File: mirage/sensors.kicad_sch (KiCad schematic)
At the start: 22 parts, among them U2 ADXL375BCCZ-RL7, U3 TMP275AIDGKR VSSOP8, U4 MS5607-02BA, U5 BMI088, U6 TMP275AIDGKR VSSOP8, U7 TMP275AIDGKR VSSOP8, U8 TMP275AIDGKR VSSOP8, U9 MMC5983MA

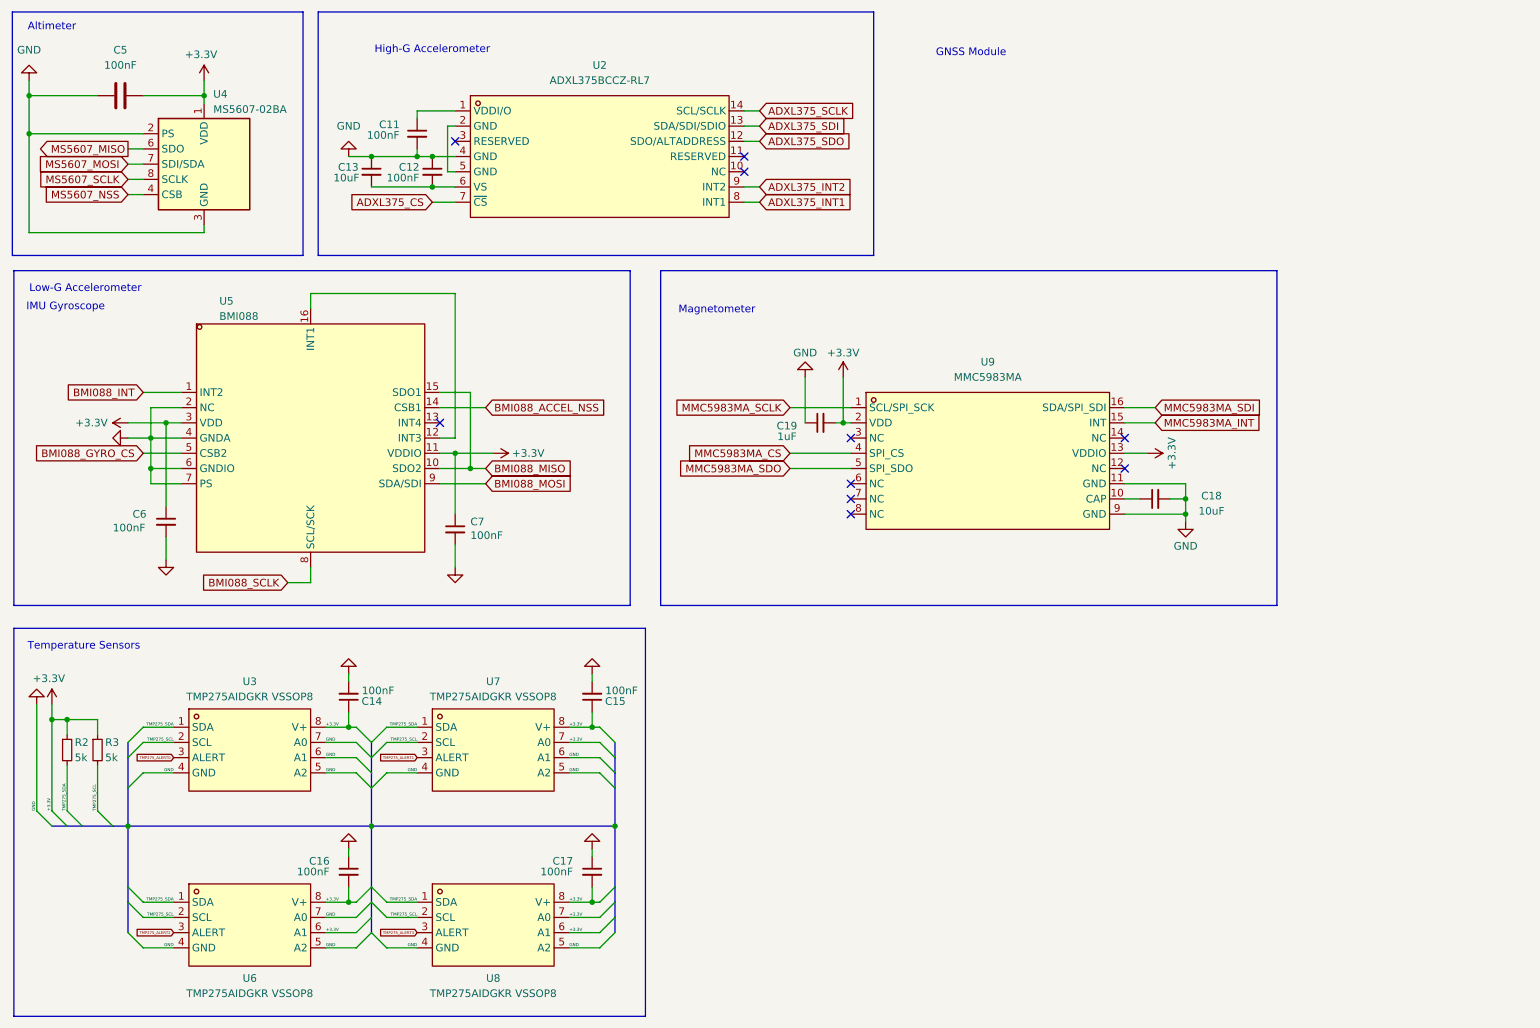
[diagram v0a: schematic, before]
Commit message: feat: connectors
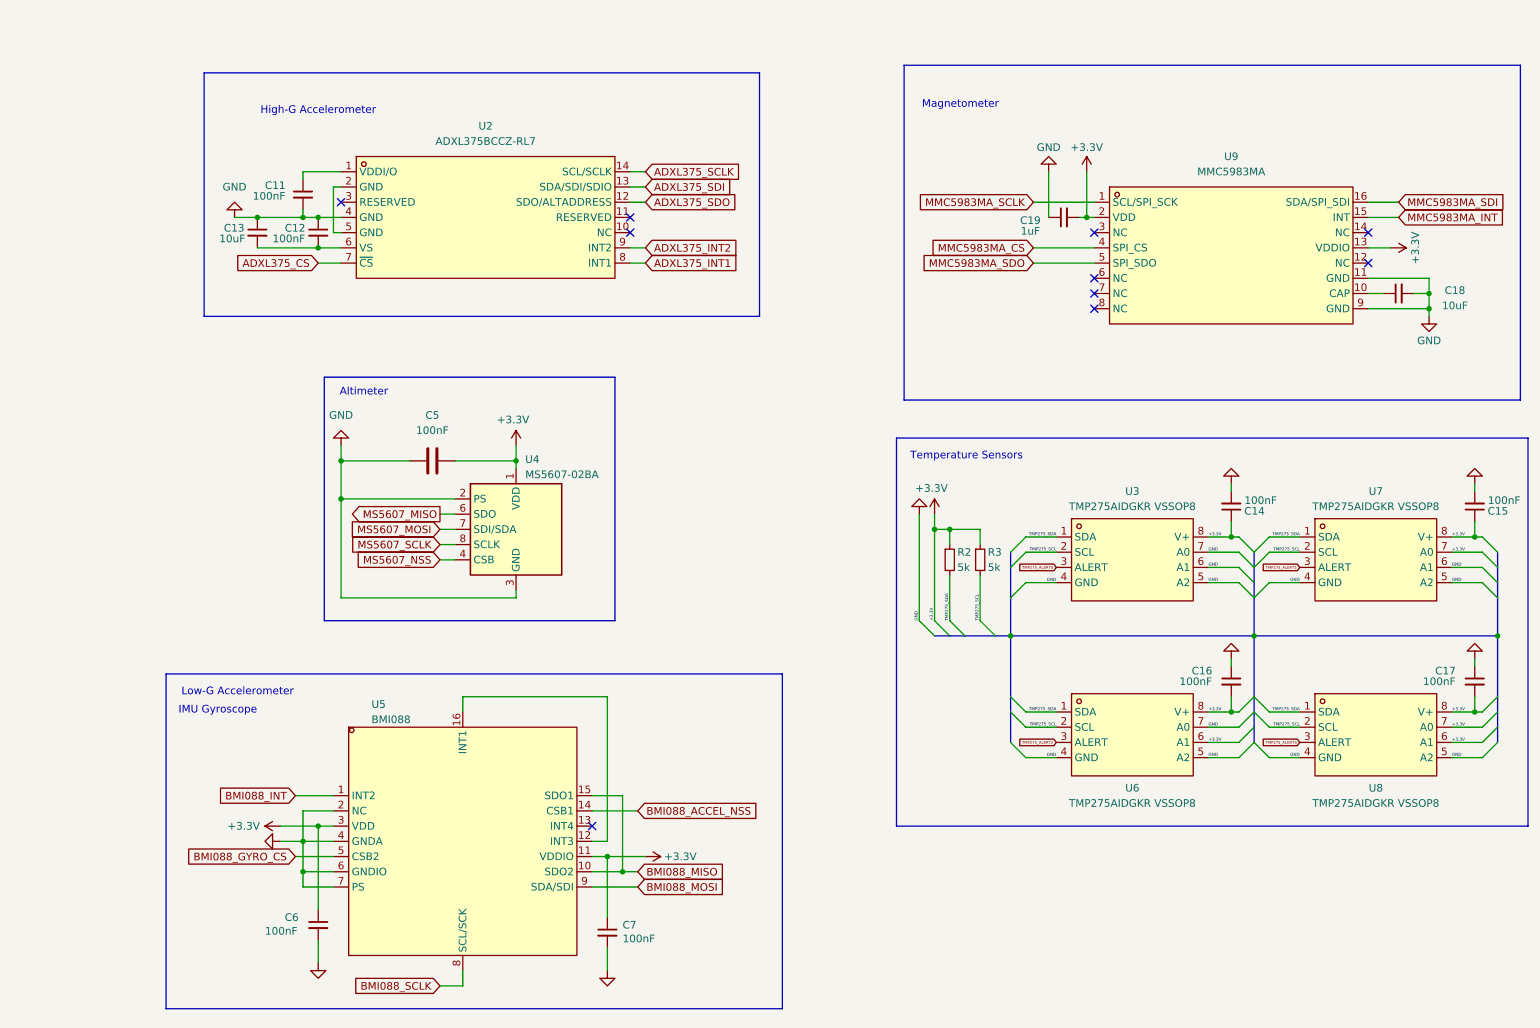
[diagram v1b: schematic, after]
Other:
- note removed: "GNSS Module"
- moved on the sheet: C11, C12, C13, C14, C15, C16, C17, C18, C19, C5, C6, C7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
